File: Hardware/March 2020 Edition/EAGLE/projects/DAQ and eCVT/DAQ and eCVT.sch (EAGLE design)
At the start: 61 parts, among them J1 5558342-1, J2 5558342-1, J3 5558342-1, J4 5558342-1, U1 AP2114H-3.3TRG1

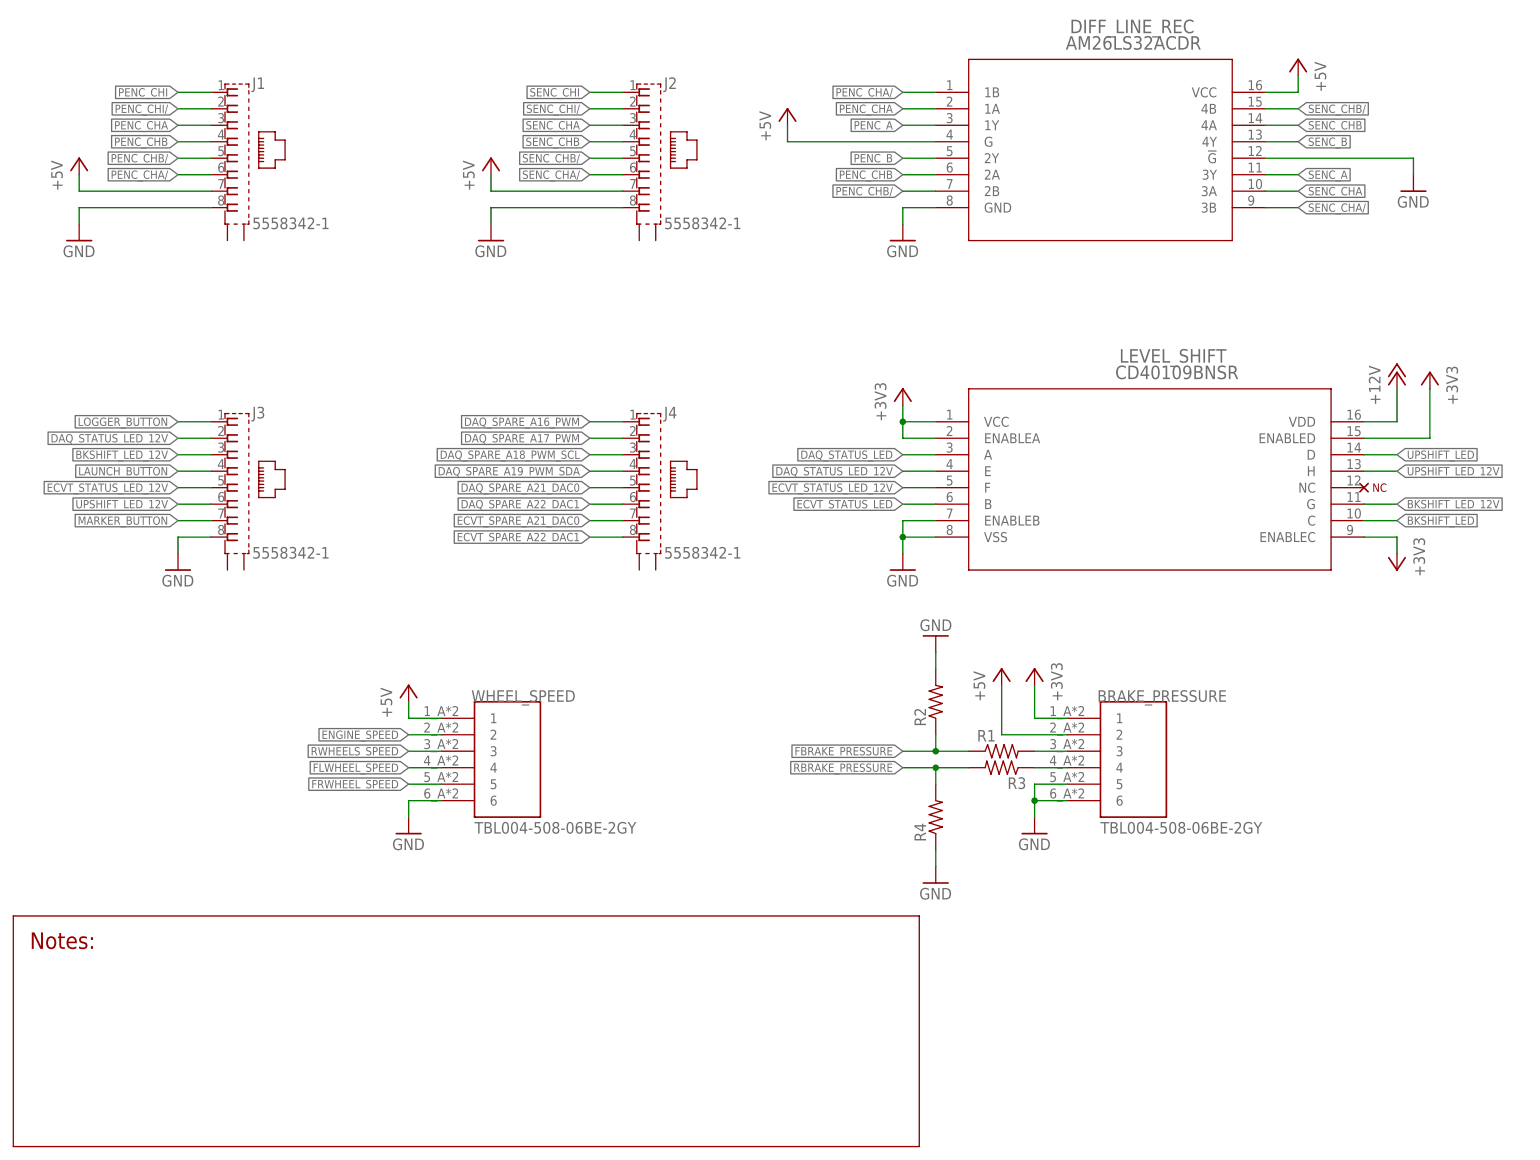
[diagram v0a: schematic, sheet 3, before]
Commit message: Almost done wiring the board!
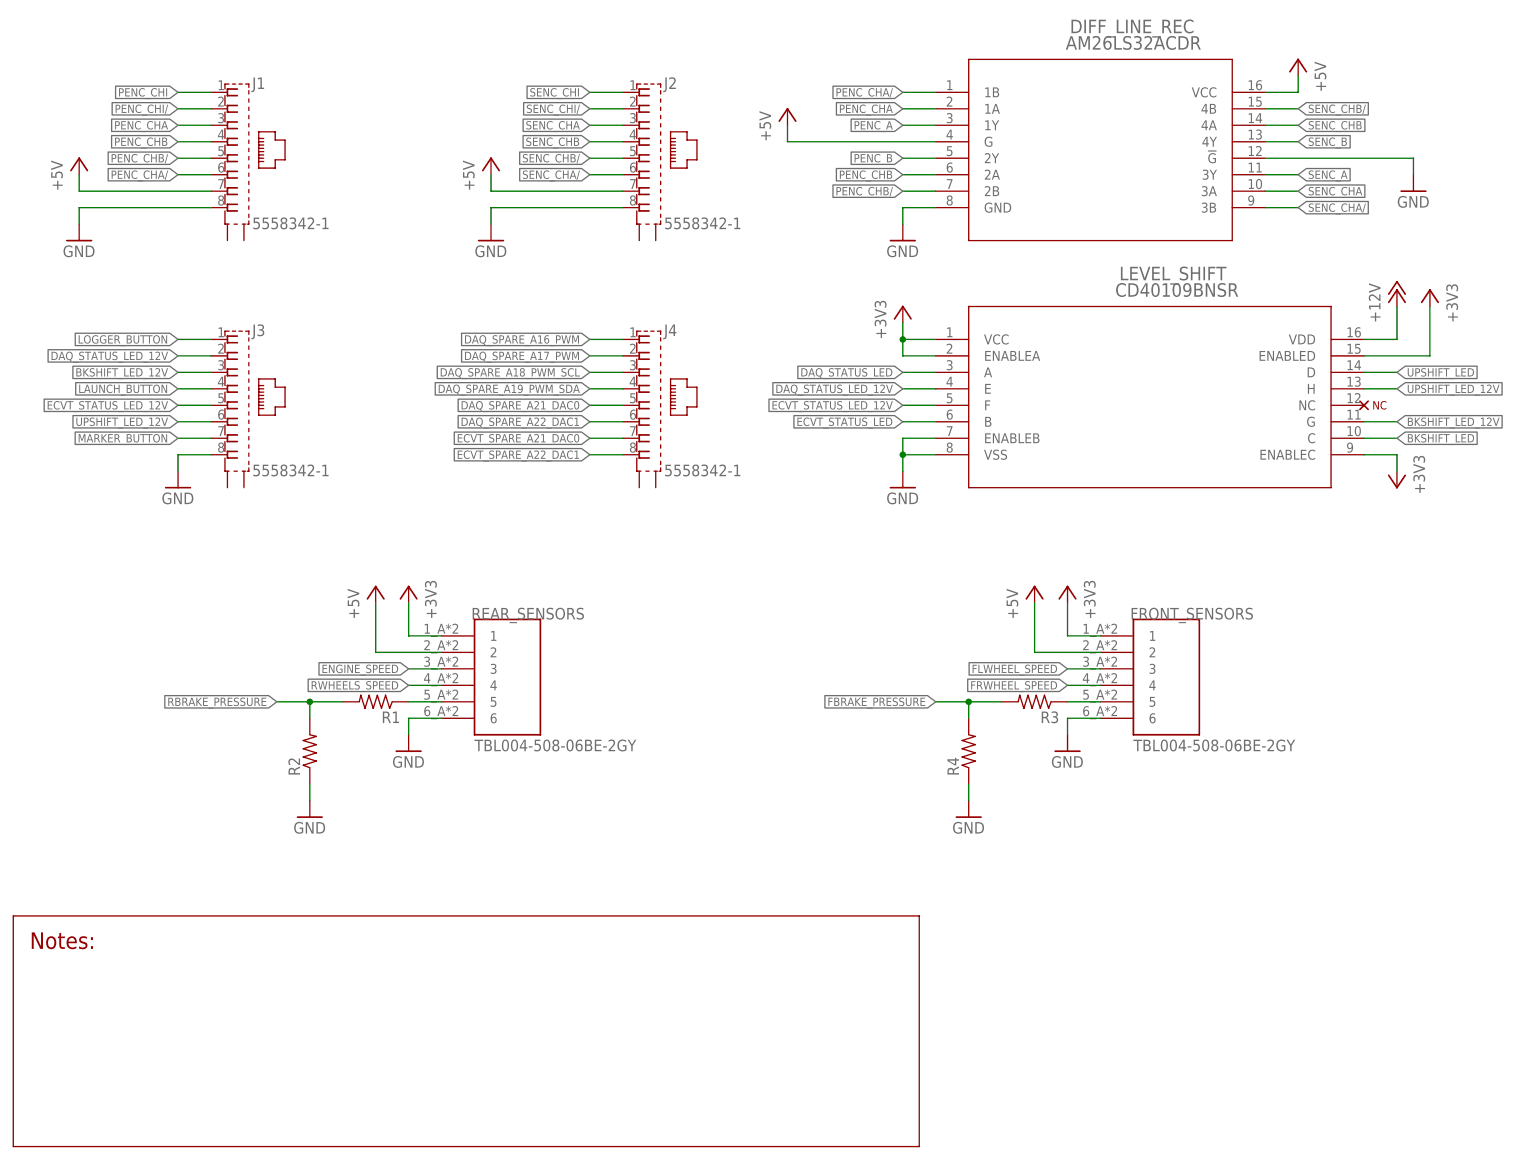
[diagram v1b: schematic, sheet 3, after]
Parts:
- removed BRAKE_PRESSURE, WHEEL_SPEED: TBL004-508-06BE-2GY, Screwless Terminal 6-Pole:TBL004-508-06BE-2GY
- added FRONT_SENSORS, REAR_SENSORS: TBL004-508-06BE-2GY, Screwless Terminal 6-Pole:TBL004-508-06BE-2GY
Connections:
- net N$1 renamed LED
- removed net FBRAKE_PRESSURE_W/O_RES: BRAKE_PRESSURE.3, R1.2
- removed net RBRAKE_PRESSURE_W/O_RES: BRAKE_PRESSURE.4, R3.1
- new net FBRAKE_PRESSURE_BEFORE_RESISTORS: FRONT_SENSORS.5, R3.1
- new net RBRAKE_PRESSURE_BEFORE_RESISTORS: R1.1, REAR_SENSORS.5
- net +3V3: now also FRONT_SENSORS.1, REAR_SENSORS.1; no longer BRAKE_PRESSURE.1
- net +5V: now also FRONT_SENSORS.2, REAR_SENSORS.2; no longer BRAKE_PRESSURE.2, WHEEL_SPEED.1
- net ENGINE_SPEED: now also REAR_SENSORS.3; no longer WHEEL_SPEED.2
- net FBRAKE_PRESSURE: now also R3.2, R4.2; no longer R1.1, R2.1
- net FLWHEEL_SPEED: now also FRONT_SENSORS.3; no longer WHEEL_SPEED.4
- net FRWHEEL_SPEED: now also FRONT_SENSORS.4; no longer WHEEL_SPEED.5
- net GND: now also FRONT_SENSORS.6, R2.1, REAR_SENSORS.6; no longer BRAKE_PRESSURE.5, BRAKE_PRESSURE.6, R2.2, WHEEL_SPEED.6
- net RBRAKE_PRESSURE: now also R1.2, R2.2; no longer R3.2, R4.2
- net RWHEELS_SPEED: now also REAR_SENSORS.4; no longer WHEEL_SPEED.3
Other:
- moved on the sheet: J3, J4, LEVEL_SHIFT, R1, R2, R3, R4

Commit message: No DRC errors! Need to do a final check + board writing
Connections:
- removed net N$19: U$33.3V3
- removed net N$2: U$31.3V3
- net +3V3: now also U$31.3V3, U$33.3V3
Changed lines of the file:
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@@
 <part name="+3V2" library="supply1" library_urn="urn:adsk.eagle:library:371" deviceset="+3V3" device=""/>
 <part name="U$22" library="ME507" deviceset="NC" device=""/>
-<part name="+3V3" library="supply1" library_urn="urn:adsk.eagle:library:371" deviceset="+3V3" device=""/>
 <part name="GND3" library="supply1" library_urn="urn:adsk.eagle:library:371" deviceset="GND" device=""/>
 <part name="GND2" library="supply1" library_urn="urn:adsk.eagle:library:371" deviceset="GND" device=""/>
@@
 <part name="+3V1" library="supply1" library_urn="urn:adsk.eagle:library:371" deviceset="+3V3" device=""/>
 <part name="U$40" library="ME507" deviceset="NC" device=""/>
-<part name="+3V4" library="supply1" library_urn="urn:adsk.eagle:library:371" deviceset="+3V3" device=""/>
 <part name="GND1" library="supply1" library_urn="urn:adsk.eagle:library:371" deviceset="GND" device=""/>
 <part name="GND5" library="supply1" library_urn="urn:adsk.eagle:library:371" deviceset="GND" device=""/>
@@
 <part name="U$31" library="Teensy" deviceset="TEENSY_3.5_BAJA" device=""/>
 <part name="U$33" library="Teensy" deviceset="TEENSY_3.5_BAJA" device=""/>
-<part name="FRAME4" library="ME 507" deviceset="TITLEBLOCK_LET_L" device=""/>
+<part name="FRAME3" library="ME 507" deviceset="TITLEBLOCK_LET_L" device=""/>
 <part name="LEVEL_SHIFT" library="Quad. Level Shifter" deviceset="CD40109BNSR" device=""/>
 <part name="P+16" library="supply1" library_urn="urn:adsk.eagle:library:371" deviceset="+12V" device=""/>
@@
 <part name="R4" library="rcl" library_urn="urn:adsk.eagle:library:334" deviceset="R-US_" device="0204/7" package3d_urn="urn:adsk.eagle:package:23498/2"/>
 <part name="R3" library="rcl" library_urn="urn:adsk.eagle:library:334" deviceset="R-US_" device="0204/7" package3d_urn="urn:adsk.eagle:package:23498/2"/>
+<part name="+3V4" library="supply1" library_urn="urn:adsk.eagle:library:371" deviceset="+3V3" device=""/>
+<part name="+3V3" library="supply1" library_urn="urn:adsk.eagle:library:371" deviceset="+3V3" device=""/>
 </parts>
 <sheets>
@@
 </instance>
 <instance part="U$22" gate="A" x="86.36" y="93.98" smashed="yes"/>
-<instance part="+3V3" gate="G$1" x="38.1" y="96.52" smashed="yes" rot="MR180">
-<attribute name="VALUE" x="35.56" y="101.6" size="1.778" layer="96" rot="MR270"/>
-</instance>
 <instance part="GND3" gate="1" x="40.64" y="142.24" smashed="yes" rot="R180">
 <attribute name="VALUE" x="43.18" y="144.78" size="1.778" layer="96" rot="R180"/>
@@
 </instance>
 <instance part="U$40" gate="A" x="200.66" y="93.98" smashed="yes"/>
-<instance part="+3V4" gate="G$1" x="134.62" y="106.68" smashed="yes">
-<attribute name="VALUE" x="132.08" y="101.6" size="1.778" layer="96" rot="R90"/>
-</instance>
 <instance part="GND1" gate="1" x="154.94" y="142.24" smashed="yes" rot="R180">
 <attribute name="VALUE" x="157.48" y="144.78" size="1.778" layer="96" rot="R180"/>
@@
 <instance part="U$31" gate="G$1" x="50.8" y="76.2" smashed="yes"/>
 <instance part="U$33" gate="G$1" x="165.1" y="76.2" smashed="yes"/>
+<instance part="+3V4" gate="G$1" x="134.62" y="106.68" smashed="yes">
+<attribute name="VALUE" x="132.08" y="101.6" size="1.778" layer="96" rot="R90"/>
+</instance>
+<instance part="+3V3" gate="G$1" x="38.1" y="96.52" smashed="yes" rot="MR180">
+<attribute name="VALUE" x="35.56" y="101.6" size="1.778" layer="96" rot="MR270"/>
+</instance>
 </instances>
 <busses>
@@
 <pinref part="U$33" gate="G$1" pin="3V3_LO"/>
 </segment>
+<segment>
+<wire x1="160.02" y1="101.6" x2="134.62" y2="101.6" width="0.1524" layer="91"/>
+<pinref part="U$33" gate="G$1" pin="3V3"/>
+<wire x1="134.62" y1="101.6" x2="134.62" y2="104.14" width="0.1524" layer="91"/>
+<pinref part="+3V4" gate="G$1" pin="+3V3"/>
+</segment>
+<segment>
+<wire x1="45.72" y1="101.6" x2="38.1" y2="101.6" width="0.1524" layer="91"/>
+<wire x1="38.1" y1="101.6" x2="38.1" y2="99.06" width="0.1524" layer="91"/>
+<pinref part="U$31" gate="G$1" pin="3V3"/>
+<pinref part="+3V3" gate="G$1" pin="+3V3"/>
+</segment>
 </net>
 <net name="DAQ_ECVT_MOSI" class="0">
@@
 </segment>
 </net>
-<net name="N$2" class="0">
-<segment>
-<wire x1="45.72" y1="101.6" x2="38.1" y2="101.6" width="0.1524" layer="91"/>
-<pinref part="+3V3" gate="G$1" pin="+3V3"/>
-<wire x1="38.1" y1="101.6" x2="38.1" y2="99.06" width="0.1524" layer="91"/>
-<pinref part="U$31" gate="G$1" pin="3V3"/>
-</segment>
-</net>
 <net name="N$3" class="0">
 <segment>
@@
 <pinref part="U$56" gate="A" pin="D"/>
 <pinref part="U$31" gate="G$1" pin="VIN"/>
-</segment>
-</net>
-<net name="N$19" class="0">
-<segment>
-<wire x1="160.02" y1="101.6" x2="134.62" y2="101.6" width="0.1524" layer="91"/>
-<pinref part="+3V4" gate="G$1" pin="+3V3"/>
-<wire x1="134.62" y1="104.14" x2="134.62" y2="101.6" width="0.1524" layer="91"/>
-<pinref part="U$33" gate="G$1" pin="3V3"/>
 </segment>
 </net>
@@
 </plain>
 <instances>
-<instance part="FRAME4" gate="G$3" x="5.08" y="0" smashed="yes"/>
-<instance part="FRAME4" gate="G$1" x="0" y="0" smashed="yes"/>
-<instance part="FRAME4" gate="G$2" x="147.32" y="0" smashed="yes">
+<instance part="FRAME3" gate="G$3" x="5.08" y="0" smashed="yes"/>
+<instance part="FRAME3" gate="G$1" x="0" y="0" smashed="yes"/>
+<instance part="FRAME3" gate="G$2" x="147.32" y="0" smashed="yes">
 <attribute name="LAST_DATE_TIME" x="160.02" y="11.43" size="2.54" layer="94"/>
 <attribute name="SHEET" x="189.23" y="6.35" size="2.54" layer="94"/>
@@
 </segment>
 </net>
-<net name="N$21" class="0">
-<segment>
-<pinref part="U$30" gate="A" pin="D"/>
-<pinref part="LEVEL_SHIFT" gate="A" pin="NC"/>
-</segment>
-</net>
 <net name="SENC_CHI" class="0">
 <segment>
@@
 </segment>
 </net>
+<net name="N$1" class="0">
+<segment>
+<pinref part="LEVEL_SHIFT" gate="A" pin="NC"/>
+<pinref part="U$30" gate="A" pin="D"/>
+</segment>
+</net>
 </nets>
 </sheet>
 </sheets>
+<errors>
+</errors>
 </schematic>
 </drawing>
